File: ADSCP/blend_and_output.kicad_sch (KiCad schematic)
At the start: 12 parts, among them J3 Output_Jack_L, J4 Output_Jack_R, U1 TL074 or OPA1644, U3 TL074 or OPA1644

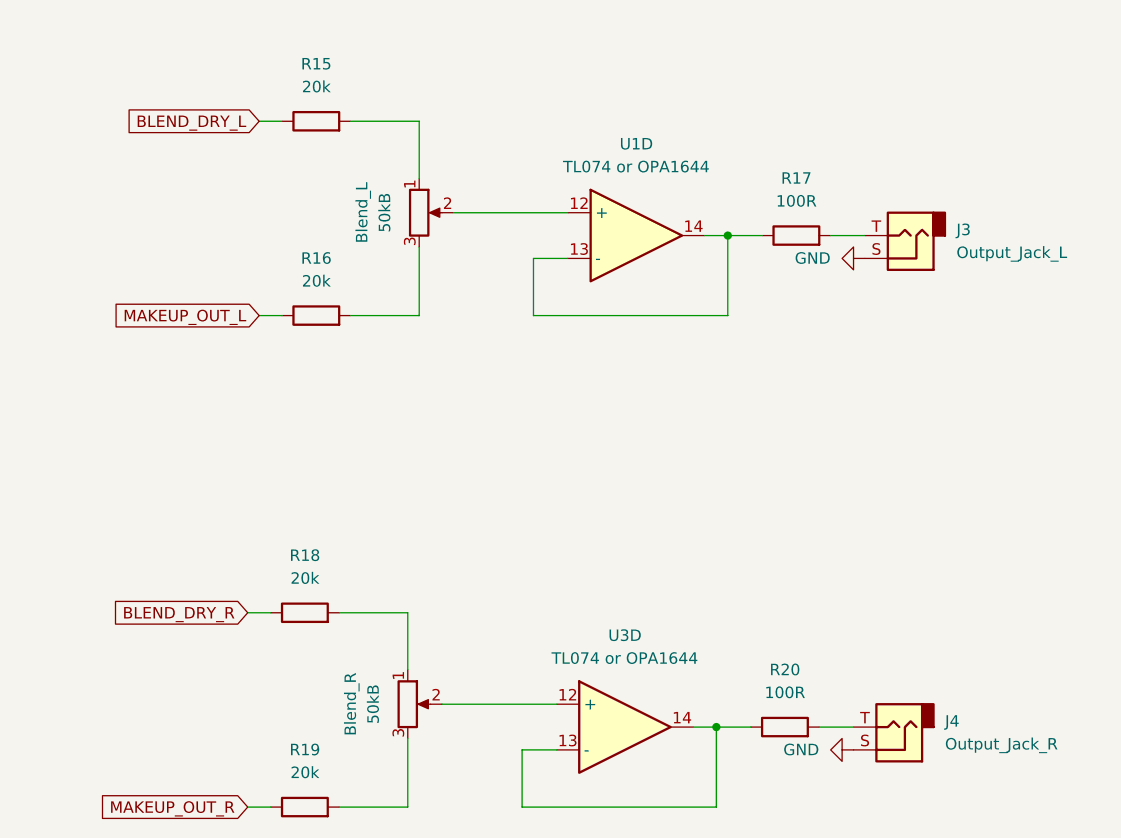
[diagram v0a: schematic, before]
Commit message: add schematics
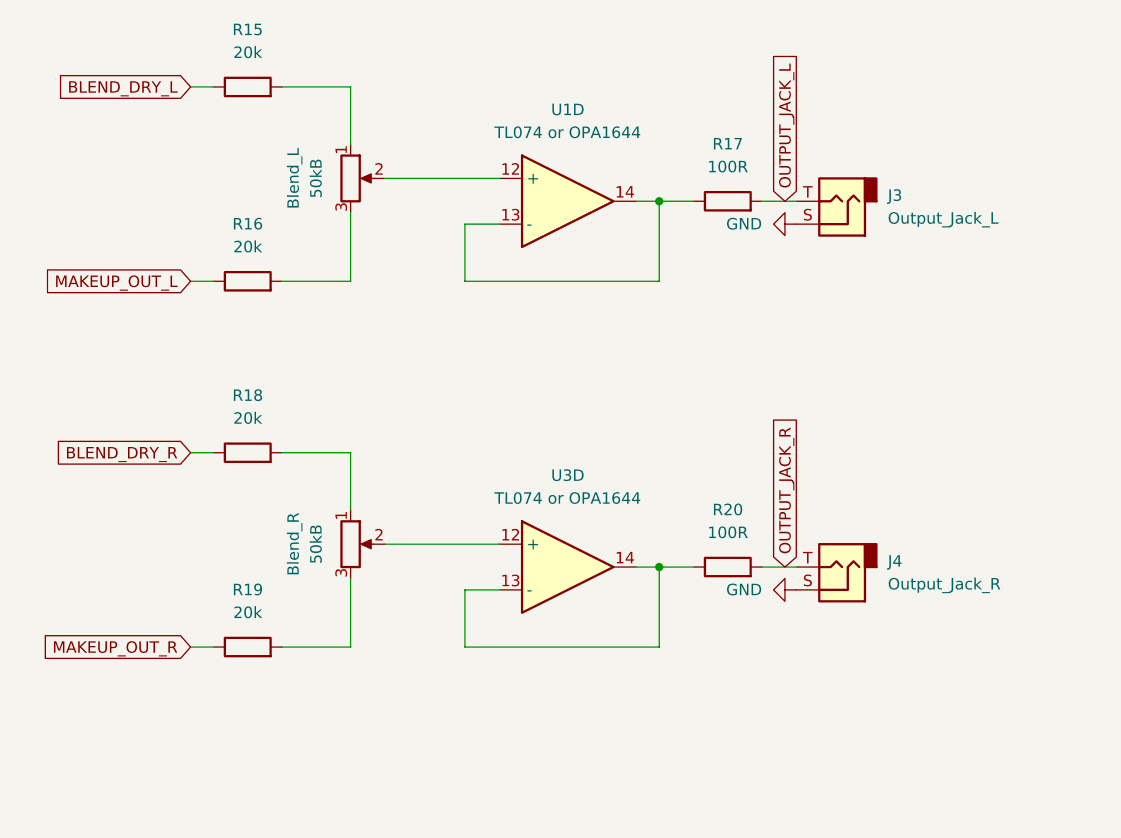
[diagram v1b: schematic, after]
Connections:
- net OUTPUT_JACK_R: now reaches J4.T, R20.2
- net OUTPUT_JACK_L: now reaches J3.T, R17.2
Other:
- moved on the sheet: Blend_L, Blend_R, J3, J4, R15, R16, R17, R18, R19, R20, U1D, U3D
